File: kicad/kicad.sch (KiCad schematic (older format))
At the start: 34 parts, among them J1 Data In, J2 Power, J3 Address Out, J4 Data Out, J5 Mode Out, SW1 SW_Push_Dual, U1 74LS374, U10 AS6C62256-70PCN, U11 SN74LS682N, U12 74LS374, U13 AT28C256-15PU, U14 SN74HC32N, U15 74LS374, U16 SN74LS682N, U17 SN74HC32N, U18 SN74154N, U2 74LS374, U3 SN74LS04N, U4 W65C02SxP, U5 74LS374, U6 74LS374, U7 SN74LS08N, U8 74LS374, U9 74LS374, X1 CXO_DIP14

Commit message: Finished schematics.
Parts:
- SW1: footprint Button_Switch_THT:SW_PUSH_6mm_H4.3mm -> Button_Switch_THT:SW_TH_Tactile_Omron_B3F-10xx
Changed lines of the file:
@@
 F 0 "SW1" V 5746 2862 50  0000 R CNN
 F 1 "SW_Push_Dual" V 5655 2862 50  0000 R CNN
-F 2 "Button_Switch_THT:SW_PUSH_6mm_H4.3mm" H 5700 3350 50  0001 C CNN
+F 2 "Button_Switch_THT:SW_TH_Tactile_Omron_B3F-10xx" H 5700 3350 50  0001 C CNN
 F 3 "~" H 5700 3350 50  0001 C CNN
 	1    5700 3150

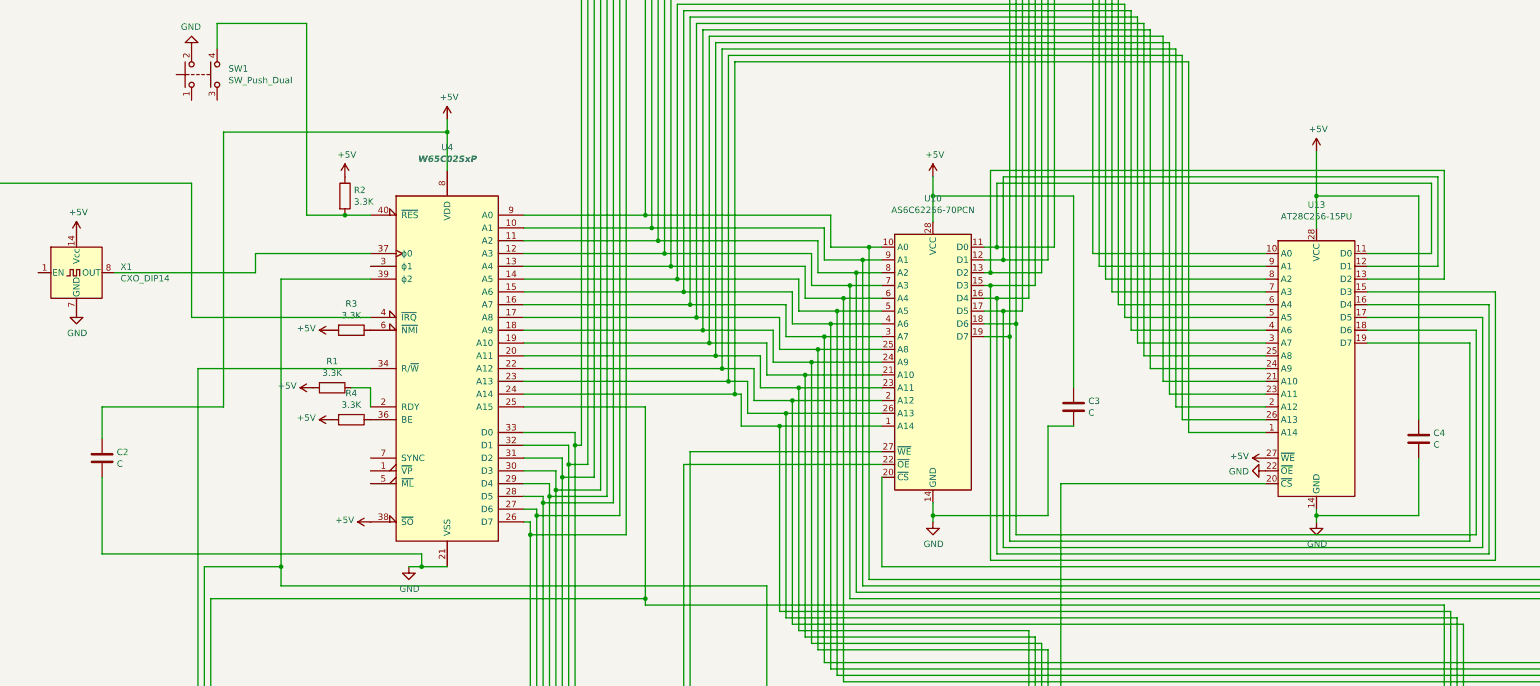
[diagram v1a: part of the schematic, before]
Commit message: Save progress on PCB.
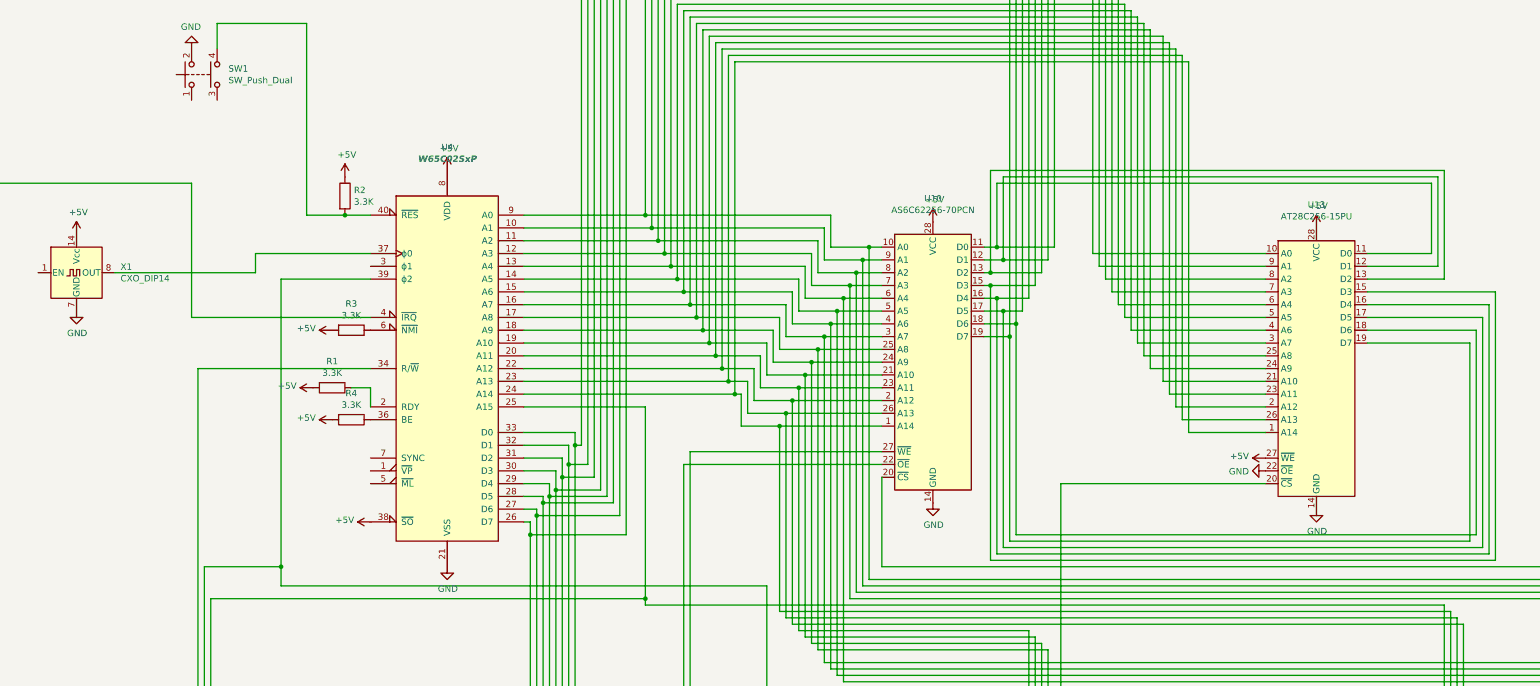
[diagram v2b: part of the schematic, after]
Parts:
- removed C2, C3, C4: C, Capacitor_THT:C_Axial_L3.8mm_D2.6mm_P7.50mm_Horizontal, symbol Device:C
- U1, U11, U12, U15, U16, U2, U5, U6, U8, U9: footprint Socket:DIP_Socket-20_W4.3_W5.08_W7.62_W10.16_W10.9_3M_220-3342-00-0602J -> Package_DIP:DIP-20_W7.62mm
- U10, U13: footprint Socket:DIP_Socket-28_W11.9_W12.7_W15.24_W17.78_W18.5_3M_228-1277-00-0602J -> Package_DIP:DIP-28_W15.24mm
- U14, U17, U3, U7: footprint Socket:DIP_Socket-14_W4.3_W5.08_W7.62_W10.16_W10.9_3M_214-3339-00-0602J -> Package_DIP:DIP-14_W7.62mm
- U18: footprint Socket:DIP_Socket-24_W11.9_W12.7_W15.24_W17.78_W18.5_3M_224-1275-00-0602J -> Package_DIP:DIP-24_W15.24mm
- U4: footprint Socket:DIP_Socket-40_W11.9_W12.7_W15.24_W17.78_W18.5_3M_240-1280-00-0602J -> Package_DIP:DIP-40_W15.24mm
